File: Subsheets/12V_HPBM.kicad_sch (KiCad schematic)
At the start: 9 parts, among them Q37 BSS123NH6327XTSA1

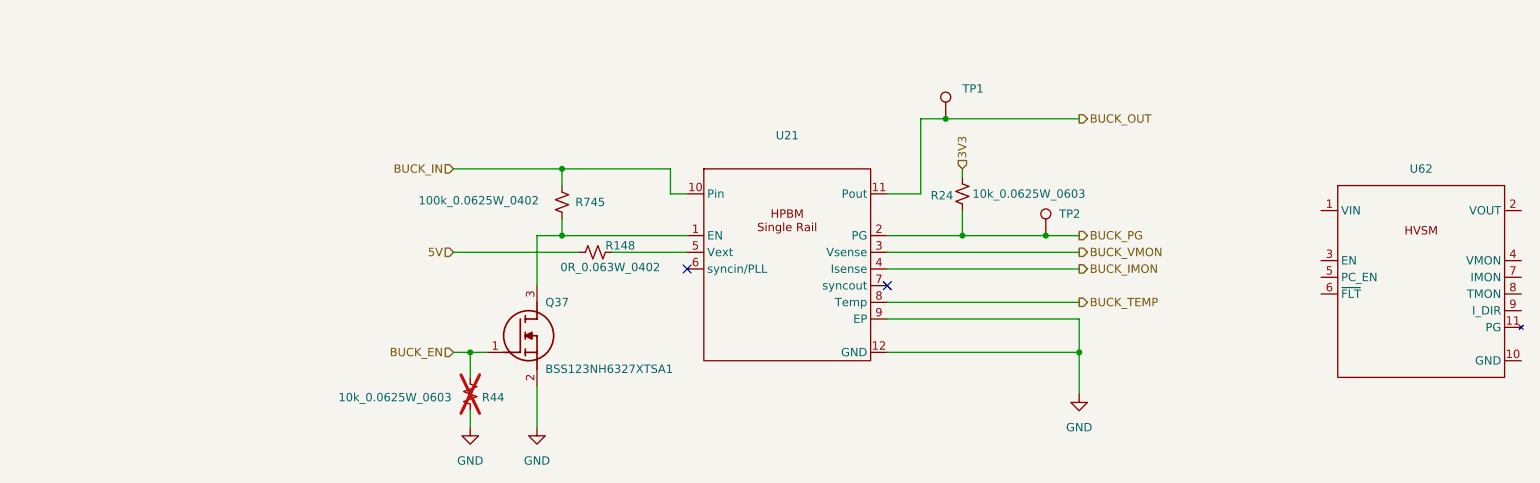
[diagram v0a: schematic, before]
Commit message: Schematic Update 1.2
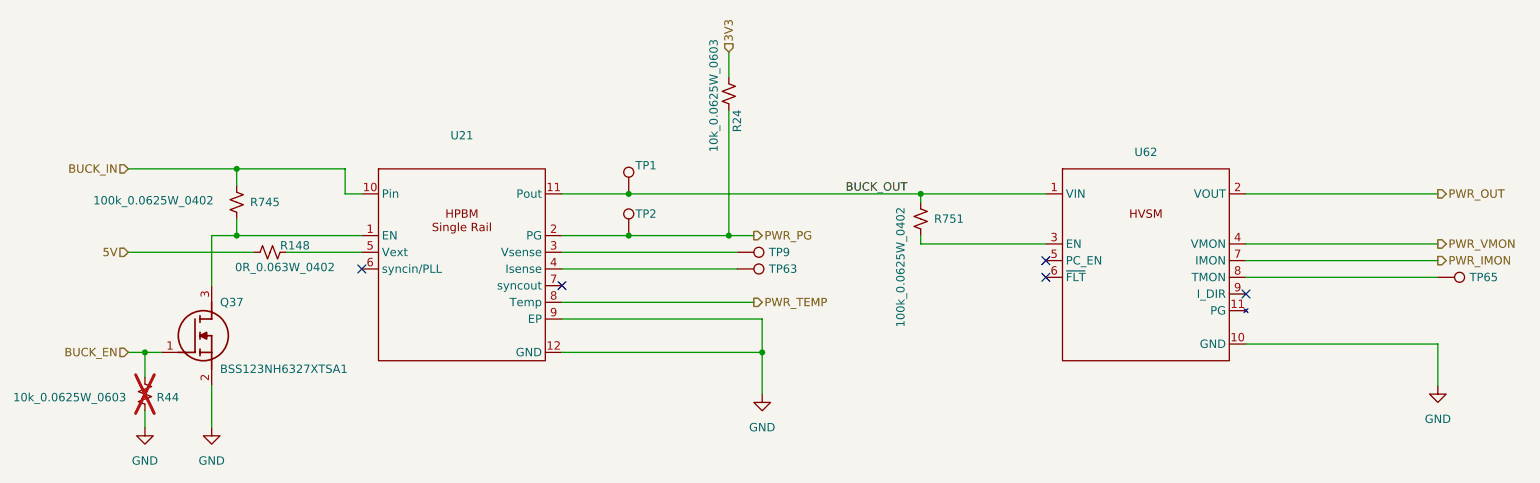
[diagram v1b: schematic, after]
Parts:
- added R751: 100k_0.0625W_0402, Pixxel_Resistors:RES0402, symbol Device:R_Small_US
- added TP63, TP65, TP9: TestPoint, symbol Connector:TestPoint
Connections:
- net BUCK_OUT: now also U62.1 (VIN), R751.2
- net GND: now also U62.10 (GND)
- net PWR_OUT: now reaches U62.2 (VOUT)
- net at U62.3 (EN): now also R751.1
- net PWR_VMON: now reaches U62.4 (VMON)
- net PWR_IMON: now reaches U62.7 (IMON)
- net at U62.8 (TMON): now also TP65.1
- net BUCK_IMON: no longer names the net of U21.4 (Isense)
- net BUCK_IMON: now also TP63.1
- net BUCK_PG renamed PWR_PG
- net BUCK_TEMP renamed PWR_TEMP
- net BUCK_VMON: no longer names the net of U21.3 (Vsense)
- net BUCK_VMON: now also TP9.1
- no-connect marks 2 -> 5
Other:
- moved on the sheet: Q37, R148, R44, R745, TP1, TP2, U21
